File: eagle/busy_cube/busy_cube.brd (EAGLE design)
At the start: 129.2 x 90.2 mm, 11 parts

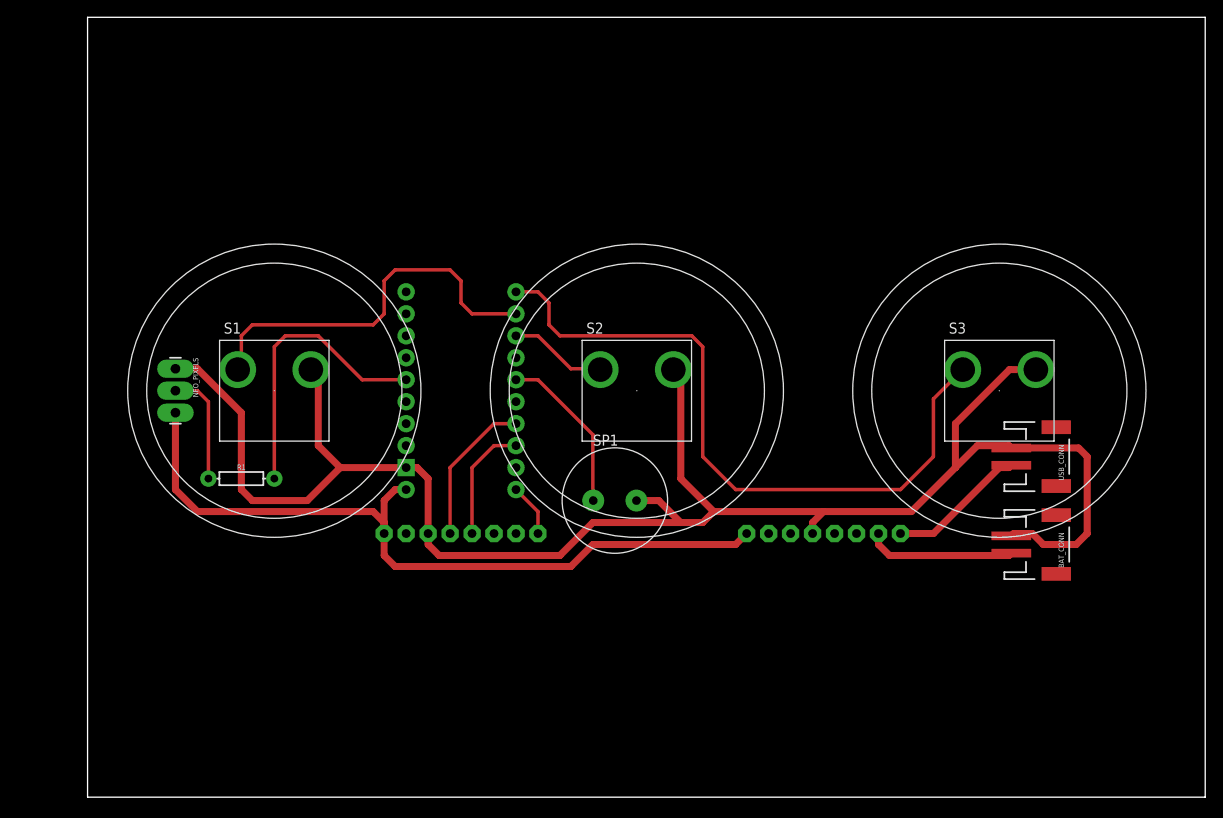
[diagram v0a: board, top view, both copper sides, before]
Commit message: some more changes
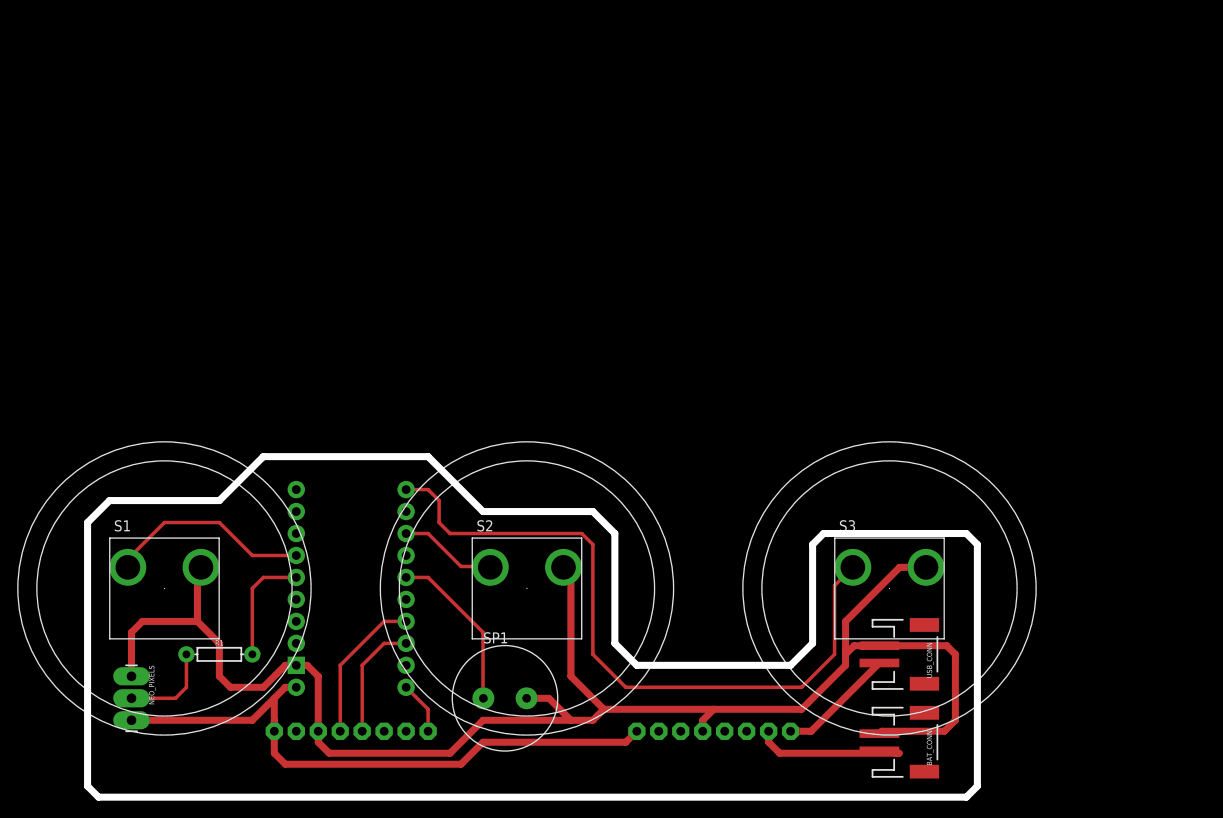
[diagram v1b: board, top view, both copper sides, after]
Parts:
- moved NEO_PIXELS 35.9 mm to (5.08, 14.0)
- moved BAT_CONN 27.5 mm to (95.2, 6.35)
- moved USB_CONN 27.5 mm to (95.2, 16.5)
- moved S1 26.2 mm to (8.89, 24.1)
- moved S2 26.2 mm to (50.8, 24.1)
- moved S3 26.2 mm to (92.7, 24.1)
- moved U$1 26.2 mm to (30.5, 24.1)
- moved LIS3DH 26.2 mm to (30.5, 7.62)
- moved POWERBOOST 26.2 mm to (72.4, 7.62)
- moved SP1 26.2 mm to (48.3, 11.4)
- moved R1 20.5 mm to (15.2, 16.5)
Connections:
- net BTN1: now also U$1.11; no longer U$1.8
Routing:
- net BTN1: track 44.8 -> 23.8 mm
- net GND: track 209.1 -> 189.0 mm
- net NEO: track 33.1 -> 13.2 mm
- net VCC: track 89.3 -> 72.3 mm
- net USB_IN_VCC: track 16.1 -> 13.5 mm
- net NEO_RES: track 13.2 -> 10.7 mm
- net BAT_IN_VCC: track 17.3 -> 19.2 mm
- net BTN3: track 79.7 -> 80.4 mm
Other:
- board size 129.2 x 90.2 mm -> 102.9 x 39.4 mm
